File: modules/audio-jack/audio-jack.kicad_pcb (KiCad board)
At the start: 2 copper layers, 17.8 x 15 mm, 6 parts, among them J1 SJ-43514-SMT-TR

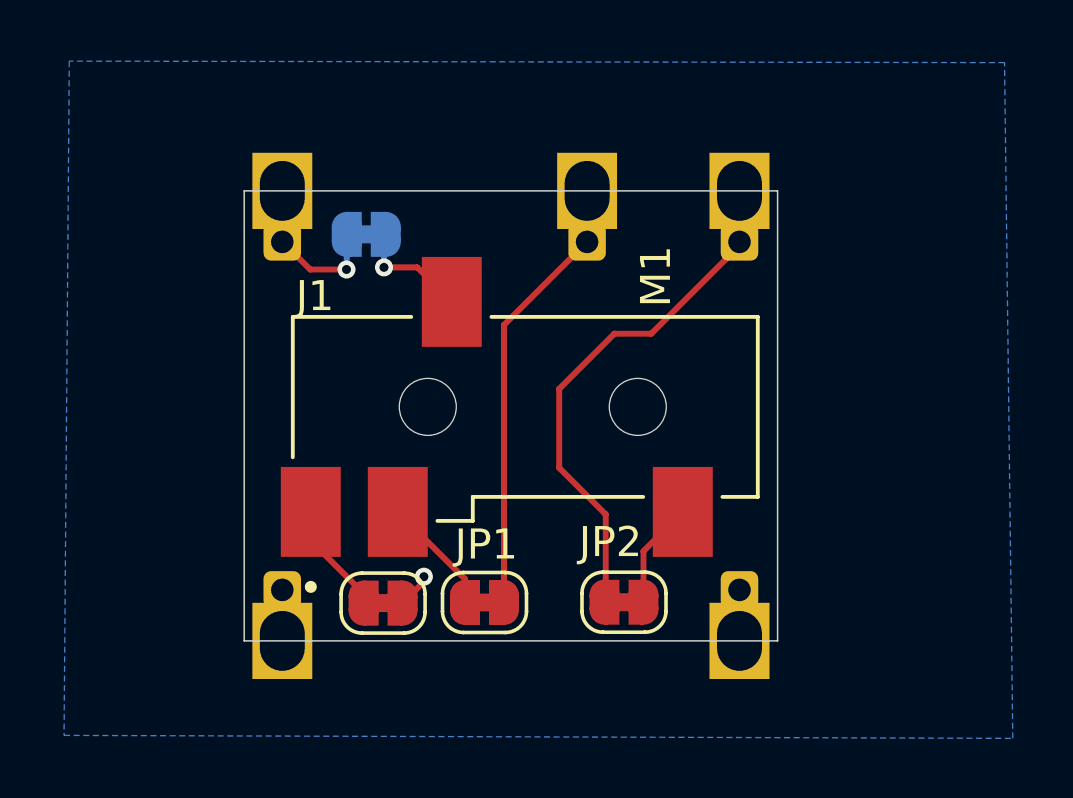
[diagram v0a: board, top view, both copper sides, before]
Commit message: Updating all modules
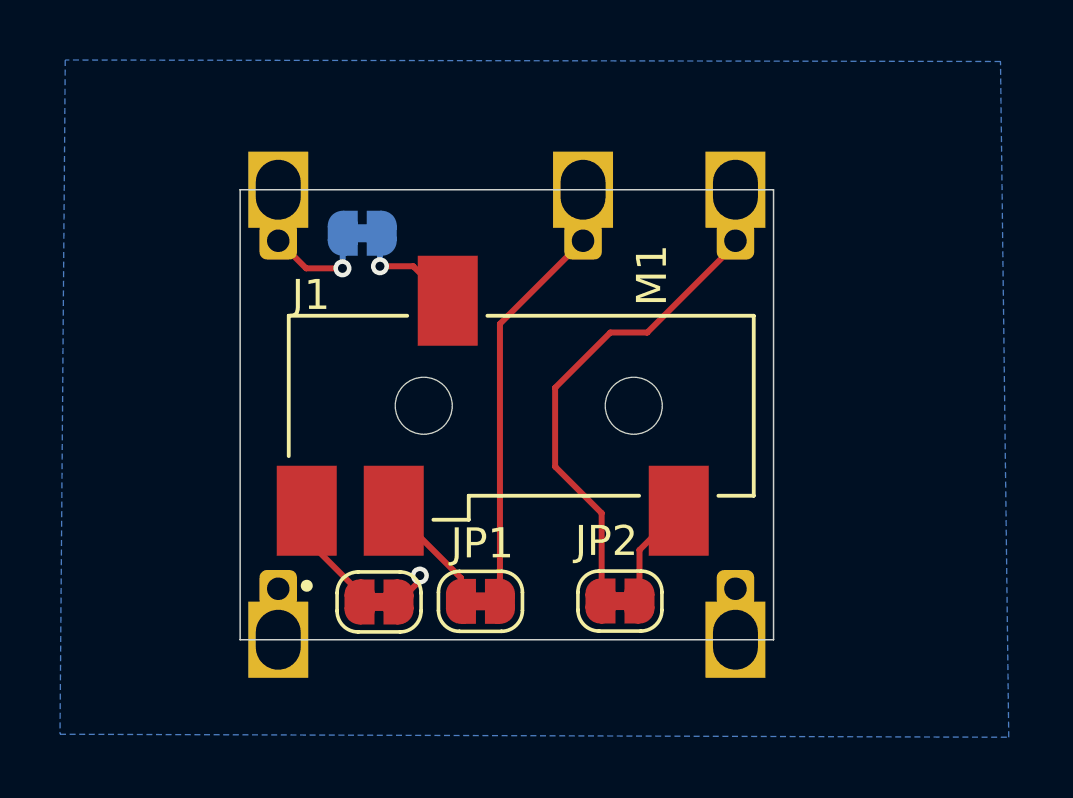
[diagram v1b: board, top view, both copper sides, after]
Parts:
- moved JP1 0.14 mm to (46.3, 43.0)
- moved JP4 0.14 mm to (42.3, 30.7)
- moved J1 0.14 mm to (40.5, 40.0)
- moved JP2 0.14 mm to (50.9, 43.0)
- moved JP3 0.14 mm to (42.9, 43.0)
- moved M1 0.14 mm to (47.1, 36.8)
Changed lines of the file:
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@@
 	(footprint "Jumper:SolderJumper-2_P1.3mm_Bridged_RoundedPad1.0x1.5mm"
 		(layer "F.Cu")
-		(at 43.01 43.04)
+		(at 42.875156 43.001969)
 		(descr "SMD Solder Jumper, 1x1.5mm, rounded Pads, 0.3mm gap, bridged with 1 copper strip")
 		(tags "net tie solder jumper bridged")
@@
 	(footprint "audio-jack:CUI_SJ-43514-SMT-TR"
 		(layer "F.Cu")
-		(at 40.6 40)
+		(at 40.465156 39.961969)
 		(property "Reference" "J1"
 			(at 0.14 -7.19 0)
@@
 	(footprint "MegaCastle:MegaCastle2x7-Module-I15.0x13.0-M8314-SPAREPAD"
 		(layer "F.Cu")
-		(at 47.27 36.8 90)
+		(at 47.135156 36.761969 90)
 		(property "Reference" "M1"
 			(at 4.65 4.84 90)
@@
 			(polygon
 				(pts
-					(xy 38.38 44.3) (xy 40.78 44.3) (xy 40.78 29.3) (xy 38.38 29.3)
+					(xy 38.245156 44.261969) (xy 40.645156 44.261969) (xy 40.645156 29.261969) (xy 38.245156 29.261969)
 				)
 			)
@@
 			(polygon
 				(pts
-					(xy 39.928592 38.784241) (xy 38.46 38.784241) (xy 38.46 34.780484) (xy 39.928592 34.780484)
+					(xy 39.793748 38.74621) (xy 38.325156 38.74621) (xy 38.325156 34.742453) (xy 39.793748 34.742453)
 				)
 			)
@@
 			(polygon
 				(pts
-					(xy 54.611408 38.784241) (xy 56.08 38.784241) (xy 56.08 34.780484) (xy 54.611408 34.780484)
+					(xy 54.476564 38.74621) (xy 55.945156 38.74621) (xy 55.945156 34.742453) (xy 54.476564 34.742453)
 				)
 			)
@@
 			(polygon
 				(pts
-					(xy 56.16 44.3) (xy 53.76 44.3) (xy 53.76 29.3) (xy 56.16 29.3)
+					(xy 56.025156 44.261969) (xy 53.625156 44.261969) (xy 53.625156 29.261969) (xy 56.025156 29.261969)
 				)
 			)
@@
 	(footprint "Jumper:SolderJumper-2_P1.3mm_Bridged_RoundedPad1.0x1.5mm"
 		(layer "F.Cu")
-		(at 51.04 43.01)
+		(at 50.905156 42.971969)
 		(descr "SMD Solder Jumper, 1x1.5mm, rounded Pads, 0.3mm gap, bridged with 1 copper strip")
 		(tags "net tie solder jumper bridged")
@@
 	(footprint "Jumper:SolderJumper-2_P1.3mm_Bridged_RoundedPad1.0x1.5mm"
 		(layer "F.Cu")
-		(at 46.39 43.02)
+		(at 46.255156 42.981969)
 		(descr "SMD Solder Jumper, 1x1.5mm, rounded Pads, 0.3mm gap, bridged with 1 copper strip")
 		(tags "net tie solder jumper bridged")
@@
 	(footprint "Jumper:SolderJumper-2_P1.3mm_Bridged_RoundedPad1.0x1.5mm"
 		(layer "B.Cu")
-		(at 42.45 30.75)
+		(at 42.315156 30.711969)
 		(descr "SMD Solder Jumper, 1x1.5mm, rounded Pads, 0.3mm gap, bridged with 1 copper strip")
 		(tags "net tie solder jumper bridged")
@@
 	)
 	(gr_text "audio-jack\nr20250219\n\n\n\ngithub.com/\ngardners/\nmegaphone-r5\n-modular"
-		(at 51.29 43.31 0)
+		(at 51.155156 43.271969 0)
 		(layer "B.SilkS")
 		(effects
@@
 	)
 	(segment
-		(start 51.69 43.01)
-		(end 51.69 41.31)
+		(start 51.555156 42.971969)
+		(end 51.555156 41.271969)
 		(width 0.2)
 		(layer "F.Cu")
@@
 	)
 	(segment
-		(start 51.69 41.31)
-		(end 53 40)
+		(start 51.555156 41.271969)
+		(end 52.865156 39.961969)
 		(width 0.2)
 		(layer "F.Cu")
@@
 	)
 	(segment
-		(start 42.36 43.04)
-		(end 42.36 42.72)
+		(start 42.225156 43.001969)
+		(end 42.225156 42.681969)
 		(width 0.2)
 		(layer "F.Cu")
@@
 	)
 	(segment
-		(start 40.6 40.96)
-		(end 40.6 40)
+		(start 40.465156 40.921969)
+		(end 40.465156 39.961969)
 		(width 0.2)
 		(layer "F.Cu")
@@
 	)
 	(segment
-		(start 42.36 42.72)
-		(end 40.6 40.96)
+		(start 42.225156 42.681969)
+		(end 40.465156 40.921969)
 		(width 0.2)
 		(layer "F.Cu")
@@
 	)
 	(segment
-		(start 43.5 40)
-		(end 45.74 42.24)
+		(start 43.365156 39.961969)
+		(end 45.605156 42.201969)
 		(width 0.2)
 		(layer "F.Cu")
@@
 	)
 	(segment
-		(start 45.74 42.24)
-		(end 45.74 43.02)
+		(start 45.605156 42.201969)
+		(end 45.605156 42.981969)
 		(width 0.2)
 		(layer "F.Cu")
@@
 	)
 	(segment
-		(start 44.15 31.85)
-		(end 43.04 31.85)
+		(start 44.015156 31.811969)
+		(end 42.905156 31.811969)
 		(width 0.2)
 		(layer "F.Cu")
@@
 	)
 	(segment
-		(start 45.3 33)
-		(end 44.15 31.85)
+		(start 45.165156 32.961969)
+		(end 44.015156 31.811969)
 		(width 0.2)
 		(layer "F.Cu")
@@
 	)
 	(via
-		(at 43.04 31.85)
+		(at 42.905156 31.811969)
 		(size 0.6)
 		(drill 0.3)
@@
 	)
 	(segment
-		(start 43.04 30.81)
-		(end 43.1 30.75)
+		(start 42.905156 30.771969)
+		(end 42.965156 30.711969)
 		(width 0.2)
 		(layer "B.Cu")
@@
 	)
 	(segment
-		(start 43.04 31.85)
-		(end 43.04 30.81)
+		(start 42.905156 31.811969)
+		(end 42.905156 30.771969)
 		(width 0.2)
 		(layer "B.Cu")
@@
 	)
 	(segment
-		(start 48.88 35.9)
-		(end 48.88 38.53)
+		(start 48.745156 35.861969)
+		(end 48.745156 38.491969)
 		(width 0.2)
 		(layer "F.Cu")
@@
 	)
 	(segment
-		(start 54.89 31)
-		(end 54.89 31.12)
+		(start 54.755156 30.961969)
+		(end 54.755156 31.081969)
 		(width 0.2)
 		(layer "F.Cu")
@@
 	)
 	(segment
-		(start 51.95 34.06)
-		(end 50.72 34.06)
+		(start 51.815156 34.021969)
+		(end 50.585156 34.021969)
 		(width 0.2)
 		(layer "F.Cu")
@@
 	)
 	(segment
-		(start 54.89 31.12)
-		(end 51.95 34.06)
+		(start 54.755156 31.081969)
+		(end 51.815156 34.021969)
 		(width 0.2)
 		(layer "F.Cu")
@@
 	)
 	(segment
-		(start 50.43 40.08)
-		(end 50.43 42.97)
+		(start 50.295156 40.041969)
+		(end 50.295156 42.931969)
 		(width 0.2)
 		(layer "F.Cu")
@@
 	)
 	(segment
-		(start 50.72 34.06)
-		(end 48.88 35.9)
+		(start 50.585156 34.021969)
+		(end 48.745156 35.861969)
 		(width 0.2)
 		(layer "F.Cu")
@@
 	)
 	(segment
-		(start 50.43 42.97)
-		(end 50.39 43.01)
+		(start 50.295156 42.931969)
+		(end 50.255156 42.971969)
 		(width 0.2)
 		(layer "F.Cu")
@@
 	)
 	(segment
-		(start 48.88 38.53)
-		(end 50.43 40.08)
+		(start 48.745156 38.491969)
+		(end 50.295156 40.041969)
 		(width 0.2)
 		(layer "F.Cu")
@@
 	)
 	(segment
-		(start 47.04 43.02)
-		(end 47.04 33.77)
+		(start 46.905156 42.981969)
+		(end 46.905156 33.731969)
 		(width 0.2)
 		(layer "F.Cu")
@@
 	)
 	(segment
-		(start 47.04 33.77)
-		(end 49.81 31)
+		(start 46.905156 33.731969)
+		(end 49.675156 30.961969)
 		(width 0.2)
 		(layer "F.Cu")
@@
 	)
 	(segment
-		(start 43.66 43.04)
-		(end 44.37 42.33)
+		(start 43.525156 43.001969)
+		(end 44.235156 42.291969)
 		(width 0.2)
 		(layer "F.Cu")
@@
 	)
 	(segment
-		(start 44.37 42.33)
-		(end 44.37 42.16)
+		(start 44.235156 42.291969)
+		(end 44.235156 42.121969)
 		(width 0.2)
 		(layer "F.Cu")
@@
 	)
 	(via
-		(at 44.37 42.16)
+		(at 44.235156 42.121969)
 		(size 0.6)
 		(drill 0.3)
@@
 	)
 	(segment
-		(start 41.79 31.92)
-		(end 40.58 31.92)
+		(start 41.655156 31.881969)
+		(end 40.445156 31.881969)
 		(width 0.2)
 		(layer "F.Cu")
@@
 	)
 	(segment
-		(start 40.58 31.92)
-		(end 39.66 31)
+		(start 40.445156 31.881969)
+		(end 39.525156 30.961969)
 		(width 0.2)
 		(layer "F.Cu")
@@
 	)
 	(segment
-		(start 39.66 31)
-		(end 39.65 31)
+		(start 39.525156 30.961969)
+		(end 39.515156 30.961969)
 		(width 0.2)
 		(layer "F.Cu")
@@
 	)
 	(via
-		(at 41.79 31.92)
+		(at 41.655156 31.881969)
 		(size 0.6)
 		(drill 0.3)
@@
 	)
 	(segment
-		(start 41.8 30.75)
-		(end 41.8 31.91)
+		(start 41.665156 30.711969)
+		(end 41.665156 31.871969)
 		(width 0.2)
 		(layer "B.Cu")
@@
 	)
 	(segment
-		(start 41.8 31.91)
-		(end 41.79 31.92)
+		(start 41.665156 31.871969)
+		(end 41.655156 31.881969)
 		(width 0.2)
 		(layer "B.Cu")
@@
 		(polygon
 			(pts
-				(xy 32.55 24.975) (xy 32.375 47.45) (xy 64 47.55) (xy 63.725 25.025)
-			)
-		)
+				(xy 32.415156 24.936969) (xy 32.240156 47.411969) (xy 63.865156 47.511969) (xy 63.590156 24.986969)
+			)
+		)
